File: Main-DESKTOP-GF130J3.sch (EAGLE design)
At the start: 87 parts, among them IC1 UCC28180D, IC2 LTV-817-B, IC3 UCC24636DBVR, Q1 CSD19531Q5AT, Q2 IPA60R330P6XKSA1, Q3 IPA65R190CFD, T1 750311798, U1 TL431SOT23, X1 6ESRM-P

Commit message: Fix Cap Size v1
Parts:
- C1: device rcl:C-EUC0402K -> rcl:C-EUC0603
- CICOMP, CVCOMP2: device rcl:C-EUC0201 -> rcl:C-EUC0603K
- CISENSE: device rcl:C-EUC0201 -> rcl:C-EUC0402
- RFBB, RFREQ1, RGATE, RGATE1, RISENSE: device rcl:R-EU_R0402 -> rcl:R-EU_R0603
- RGATE2, RVCOMP: device rcl:R-EU_R0201 -> rcl:R-EU_R0603
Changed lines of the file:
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@@
 <part name="COUT" library="cap-pan40" deviceset="C-NP" device="-10,0-14,0X6,0" value="5.435mF"/>
 <part name="DSTART" library="diode" library_urn="urn:adsk.eagle:library:210" deviceset="1N4446" device="" package3d_urn="urn:adsk.eagle:package:43344/2"/>
-<part name="RGATE1" library="rcl" library_urn="urn:adsk.eagle:library:334" deviceset="R-EU_" device="R0402" package3d_urn="urn:adsk.eagle:package:23547/3" value="1.07"/>
-<part name="RGATE2" library="rcl" library_urn="urn:adsk.eagle:library:334" deviceset="R-EU_" device="R0201" package3d_urn="urn:adsk.eagle:package:26117/2" value="10K"/>
+<part name="RGATE1" library="rcl" library_urn="urn:adsk.eagle:library:334" deviceset="R-EU_" device="R0603" package3d_urn="urn:adsk.eagle:package:23555/3" value="1.07"/>
+<part name="RGATE2" library="rcl" library_urn="urn:adsk.eagle:library:334" deviceset="R-EU_" device="R0603" package3d_urn="urn:adsk.eagle:package:23555/3" value="10K"/>
 <part name="IC1" library="SamacSys_Parts" deviceset="UCC28180D" device=""/>
 <part name="PGND" library="supply1" library_urn="urn:adsk.eagle:library:371" deviceset="GND" device="" value="PGND"/>
 <part name="CVSENSE" library="rcl" library_urn="urn:adsk.eagle:library:334" deviceset="C-EU" device="C0805" package3d_urn="urn:adsk.eagle:package:23617/2" value="820nF"/>
-<part name="CICOMP" library="rcl" library_urn="urn:adsk.eagle:library:334" deviceset="C-EU" device="C0201" package3d_urn="urn:adsk.eagle:package:23690/2" value="1.5nF"/>
-<part name="RISENSE" library="rcl" library_urn="urn:adsk.eagle:library:334" deviceset="R-EU_" device="R0402" package3d_urn="urn:adsk.eagle:package:23547/3" value="221"/>
+<part name="CICOMP" library="rcl" library_urn="urn:adsk.eagle:library:334" deviceset="C-EU" device="C0603K" package3d_urn="urn:adsk.eagle:package:23680/2" value="1.5nF"/>
+<part name="RISENSE" library="rcl" library_urn="urn:adsk.eagle:library:334" deviceset="R-EU_" device="R0603" package3d_urn="urn:adsk.eagle:package:23555/3" value="221"/>
 <part name="VBULK" library="supply2" library_urn="urn:adsk.eagle:library:372" deviceset="VPP" device=""/>
-<part name="RFREQ1" library="rcl" library_urn="urn:adsk.eagle:library:334" deviceset="R-EU_" device="R0402" package3d_urn="urn:adsk.eagle:package:23547/3" value="17.4K"/>
+<part name="RFREQ1" library="rcl" library_urn="urn:adsk.eagle:library:334" deviceset="R-EU_" device="R0603" package3d_urn="urn:adsk.eagle:package:23555/3" value="17.4K"/>
 <part name="L5" library="Wurth_Elektronik_Passive_rev18f" library_urn="urn:adsk.eagle:library:7584915" deviceset="WE-FI" device="_7447016" package3d_urn="urn:adsk.eagle:package:7586765/3"/>
 <part name="L6" library="Wurth_Elektronik_Passive_rev18f" library_urn="urn:adsk.eagle:library:7584915" deviceset="WE-FI" device="_7447016" package3d_urn="urn:adsk.eagle:package:7586765/3"/>
 <part name="DBOOST" library="diode" library_urn="urn:adsk.eagle:library:210" deviceset="DIODE-" device="TO220V" package3d_urn="urn:adsk.eagle:package:43373/3" value="LXA06T600"/>
 <part name="Q2" library="transistor-power" library_urn="urn:adsk.eagle:library:400" deviceset="PMOSFET_N" device="TO220BV" package3d_urn="urn:adsk.eagle:package:29484/3" value="IPA60R330P6XKSA1"/>
-<part name="CISENSE" library="rcl" library_urn="urn:adsk.eagle:library:334" deviceset="C-EU" device="C0201" package3d_urn="urn:adsk.eagle:package:23690/2" value="1nF"/>
+<part name="CISENSE" library="rcl" library_urn="urn:adsk.eagle:library:334" deviceset="C-EU" device="C0402" package3d_urn="urn:adsk.eagle:package:23626/2" value="1nF"/>
 <part name="CVCOMP" library="rcl" library_urn="urn:adsk.eagle:library:334" deviceset="C-EU" device="C0805" package3d_urn="urn:adsk.eagle:package:23617/2" value="22uF"/>
 <part name="SUPPLY2" library="supply2" library_urn="urn:adsk.eagle:library:372" deviceset="GND" device="" value="PGND"/>
 <part name="DTURNOFF" library="SamacSys_Parts" deviceset="MBR0540T1G" device=""/>
-<part name="RFBB" library="rcl" library_urn="urn:adsk.eagle:library:334" deviceset="R-EU_" device="R0402" package3d_urn="urn:adsk.eagle:package:23547/3" value="13K"/>
-<part name="RGATE" library="rcl" library_urn="urn:adsk.eagle:library:334" deviceset="R-EU_" device="R0402" package3d_urn="urn:adsk.eagle:package:23547/3" value="3.92"/>
-<part name="C1" library="rcl" library_urn="urn:adsk.eagle:library:334" deviceset="C-EU" device="C0402K" package3d_urn="urn:adsk.eagle:package:23679/2" value="100nF"/>
+<part name="RFBB" library="rcl" library_urn="urn:adsk.eagle:library:334" deviceset="R-EU_" device="R0603" package3d_urn="urn:adsk.eagle:package:23555/3" value="13K"/>
+<part name="RGATE" library="rcl" library_urn="urn:adsk.eagle:library:334" deviceset="R-EU_" device="R0603" package3d_urn="urn:adsk.eagle:package:23555/3" value="3.92"/>
+<part name="C1" library="rcl" library_urn="urn:adsk.eagle:library:334" deviceset="C-EU" device="C0603" package3d_urn="urn:adsk.eagle:package:23616/2" value="100nF"/>
 <part name="RSENSE" library="ERJ-L03KF50MV" deviceset="ERJ-L03KF50MV" device=""/>
 <part name="RFBT" library="CRCW2512300KJNEG" deviceset="CRCW2512300KJNEG" device=""/>
 <part name="RFBT1" library="CRCW2512300KJNEG" deviceset="CRCW2512300KJNEG" device=""/>
 <part name="RFBT2" library="CRCW2512402KFKEG" deviceset="CRCW2512402KFKEG" device=""/>
-<part name="CVCOMP2" library="rcl" library_urn="urn:adsk.eagle:library:334" deviceset="C-EU" device="C0201" package3d_urn="urn:adsk.eagle:package:23690/2" value="22nF"/>
-<part name="RVCOMP" library="rcl" library_urn="urn:adsk.eagle:library:334" deviceset="R-EU_" device="R0201" package3d_urn="urn:adsk.eagle:package:26117/2" value="287K"/>
+<part name="CVCOMP2" library="rcl" library_urn="urn:adsk.eagle:library:334" deviceset="C-EU" device="C0603K" package3d_urn="urn:adsk.eagle:package:23680/2" value="22nF"/>
+<part name="RVCOMP" library="rcl" library_urn="urn:adsk.eagle:library:334" deviceset="R-EU_" device="R0603" package3d_urn="urn:adsk.eagle:package:23555/3" value="287K"/>
 <part name="COUTX" library="cap-pan40" deviceset="C-NP" device="-10,0-14,0X6,0" value="100nF"/>
 <part name="DZ" library="TZMC1V0-M-18" deviceset="TZMC1V0-M-18" device="" package3d_urn="urn:adsk.eagle:package:11886536/1"/>

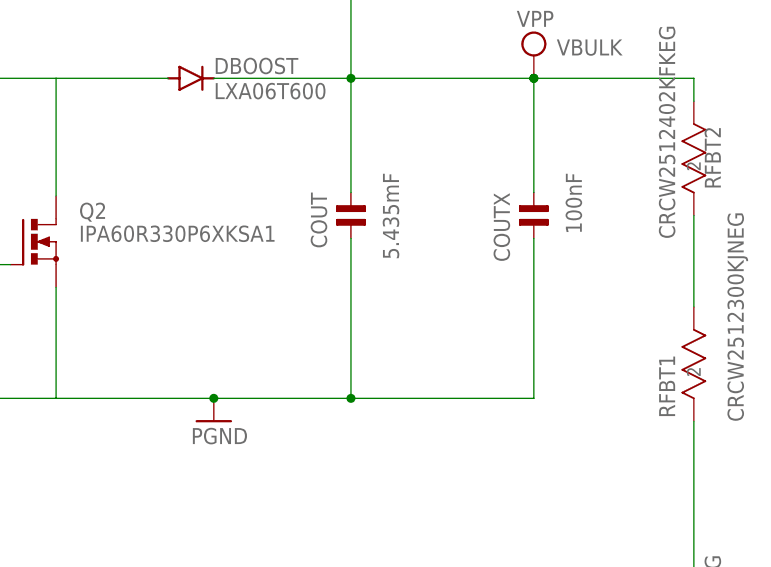
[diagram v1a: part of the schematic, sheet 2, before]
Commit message: Cav Size v2
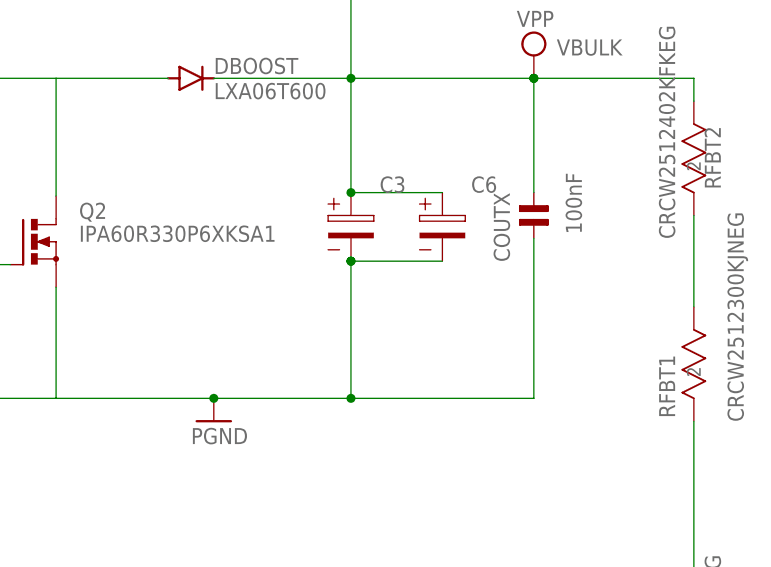
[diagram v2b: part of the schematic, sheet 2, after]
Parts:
- removed COUT: 5.435mF, cap-pan40:C-NP-10,0-14,0X6,0
- added C3, C6: (no value), Wurth_Elektronik_Passive_Capacitors_rev18b:WCAP-AIG8_30X46_861011485018
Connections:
- net GND: now also C3.2, C6.2; no longer COUT.2
- net VBULK: now also C3.1, C6.1; no longer COUT.1
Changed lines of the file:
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@@
 <part name="Q1" library="SamacSys_Parts" deviceset="CSD19531Q5AT" device=""/>
 <part name="LBST" library="Wurth_Elektronik_Passive_rev18f" library_urn="urn:adsk.eagle:library:7584915" deviceset="WE-SI" device="_744139" package3d_urn="urn:adsk.eagle:package:7586520/3" value="494.23uH"/>
-<part name="COUT" library="cap-pan40" deviceset="C-NP" device="-10,0-14,0X6,0" value="5.435mF"/>
 <part name="DSTART" library="diode" library_urn="urn:adsk.eagle:library:210" deviceset="1N4446" device="" package3d_urn="urn:adsk.eagle:package:43344/2"/>
 <part name="RGATE1" library="rcl" library_urn="urn:adsk.eagle:library:334" deviceset="R-EU_" device="R0603" package3d_urn="urn:adsk.eagle:package:23555/3" value="1.07"/>
@@
 <part name="CIN" library="rcl" library_urn="urn:adsk.eagle:library:334" deviceset="C-EU" device="150-072X183" package3d_urn="urn:adsk.eagle:package:23657/1" value="890283325008CS"/>
 <part name="B2" library="rectifier" library_urn="urn:adsk.eagle:library:336" deviceset="GBU4" device="" package3d_urn="urn:adsk.eagle:package:23875/1"/>
+<part name="C3" library="Wurth_Elektronik_Passive_Capacitors_rev18b" library_urn="urn:adsk.eagle:library:491551" deviceset="WCAP-AIG8" device="_861011485018" package3d_urn="urn:adsk.eagle:package:491739/2" technology="_30X46"/>
+<part name="C6" library="Wurth_Elektronik_Passive_Capacitors_rev18b" library_urn="urn:adsk.eagle:library:491551" deviceset="WCAP-AIG8" device="_861011485018" package3d_urn="urn:adsk.eagle:package:491739/2" technology="_30X46"/>
 </parts>
 <sheets>
@@
 <attribute name="VALUE" x="55.88" y="88.9" size="1.778" layer="96"/>
 </instance>
-<instance part="COUT" gate="G$1" x="132.08" y="76.2" smashed="yes" rot="R270">
-<attribute name="NAME" x="127.635" y="78.74" size="1.778" layer="95" rot="R270"/>
-<attribute name="VALUE" x="135.636" y="80.9625" size="1.778" layer="96" rot="R270"/>
-</instance>
 <instance part="DSTART" gate="1" x="73.66" y="101.6" smashed="yes">
 <attribute name="NAME" x="76.2" y="102.0826" size="1.778" layer="95"/>
@@
 <attribute name="NAME" x="10.16" y="93.98" size="1.778" layer="95"/>
 <attribute name="VALUE" x="10.16" y="87.63" size="1.778" layer="96"/>
+</instance>
+<instance part="C3" gate="G$1" x="132.08" y="73.66" smashed="yes">
+<attribute name="NAME" x="135.255" y="78.74" size="1.778" layer="95"/>
+<attribute name="VALUE" x="135.255" y="70.485" size="1.778" layer="96"/>
+</instance>
+<instance part="C6" gate="G$1" x="142.24" y="73.66" smashed="yes">
+<attribute name="NAME" x="145.415" y="78.74" size="1.778" layer="95"/>
+<attribute name="VALUE" x="145.415" y="70.485" size="1.778" layer="96"/>
 </instance>
 </instances>
@@
 <pinref part="DSTART" gate="1" pin="C"/>
 <wire x1="76.2" y1="101.6" x2="132.08" y2="101.6" width="0.1524" layer="91"/>
-<pinref part="COUT" gate="G$1" pin="1"/>
 <wire x1="132.08" y1="78.74" x2="132.08" y2="91.44" width="0.1524" layer="91"/>
 <wire x1="116.84" y1="91.44" x2="132.08" y2="91.44" width="0.1524" layer="91"/>
@@
 <pinref part="RFBT2" gate="A" pin="1"/>
 <wire x1="170.18" y1="91.44" x2="170.18" y2="88.9" width="0.1524" layer="91"/>
+<pinref part="C3" gate="G$1" pin="1"/>
+<junction x="132.08" y="78.74"/>
+<pinref part="C6" gate="G$1" pin="1"/>
+<wire x1="142.24" y1="78.74" x2="132.08" y2="78.74" width="0.1524" layer="91"/>
 </segment>
 </net>
@@
 <net name="GND" class="0">
 <segment>
-<pinref part="COUT" gate="G$1" pin="2"/>
-<wire x1="132.08" y1="55.88" x2="132.08" y2="73.66" width="0.1524" layer="91"/>
+<wire x1="132.08" y1="55.88" x2="132.08" y2="71.12" width="0.1524" layer="91"/>
 <wire x1="116.84" y1="55.88" x2="132.08" y2="55.88" width="0.1524" layer="91"/>
 <pinref part="PGND" gate="1" pin="GND"/>
@@
 <pinref part="COUTX" gate="G$1" pin="2"/>
 <wire x1="152.4" y1="55.88" x2="152.4" y2="73.66" width="0.1524" layer="91"/>
-</segment>
-</net>
+<junction x="132.08" y="71.12"/>
+<pinref part="C3" gate="G$1" pin="2"/>
+<junction x="132.08" y="71.12"/>
+<pinref part="C6" gate="G$1" pin="2"/>
+<wire x1="132.08" y1="71.12" x2="142.24" y2="71.12" width="0.1524" layer="91"/>
+</segment>
+</net>
